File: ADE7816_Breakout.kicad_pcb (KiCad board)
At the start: 2 copper layers, 66 x 76.2 mm, 56 parts, among them J1 AudioJack3, J2 AudioJack3, J3 AudioJack3, J4 AudioJack3, J5 AudioJack3, J6 AudioJack3, J7 Barrel_Jack_Switch, J8 Conn_01x10, U1 ADE7816ACPZ, Y1 16.384MHz

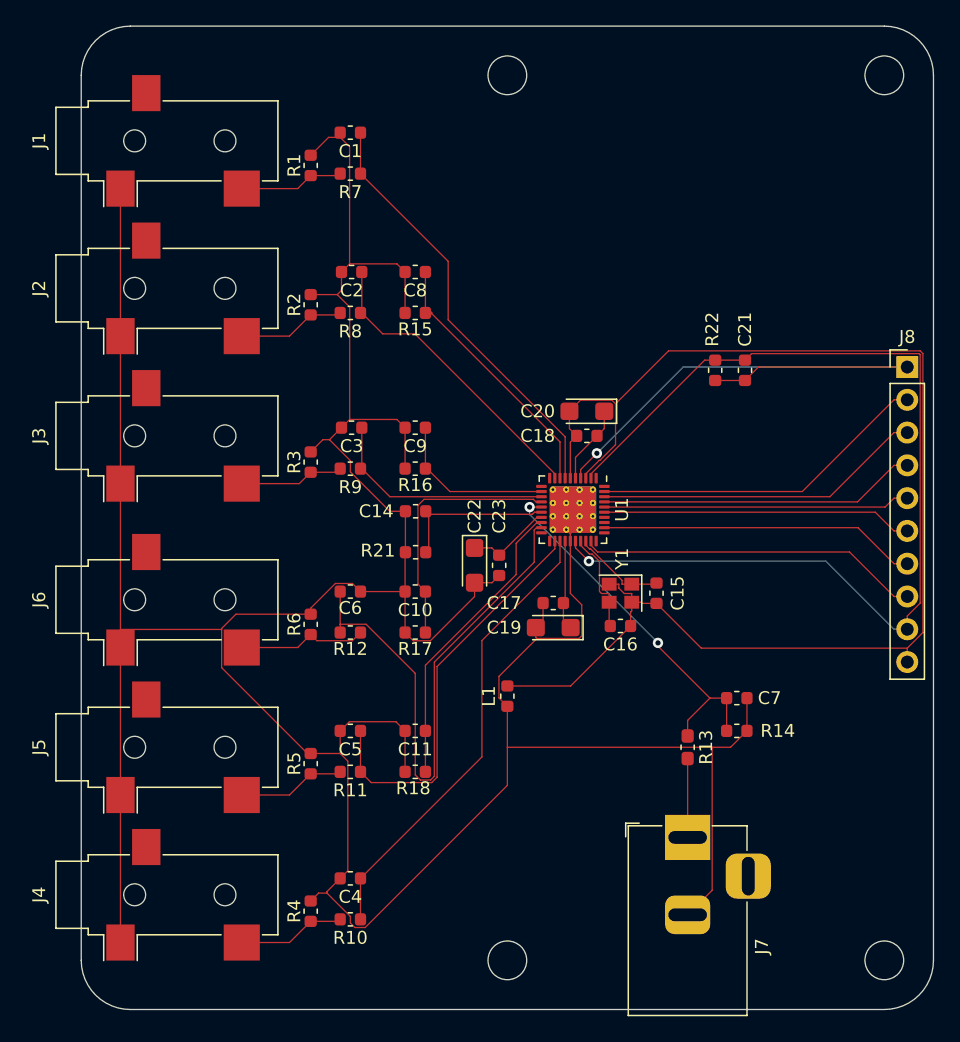
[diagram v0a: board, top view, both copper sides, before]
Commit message: Some routing
Signed-off-by: Tisham Dhar <whatnickd@gmail.com>
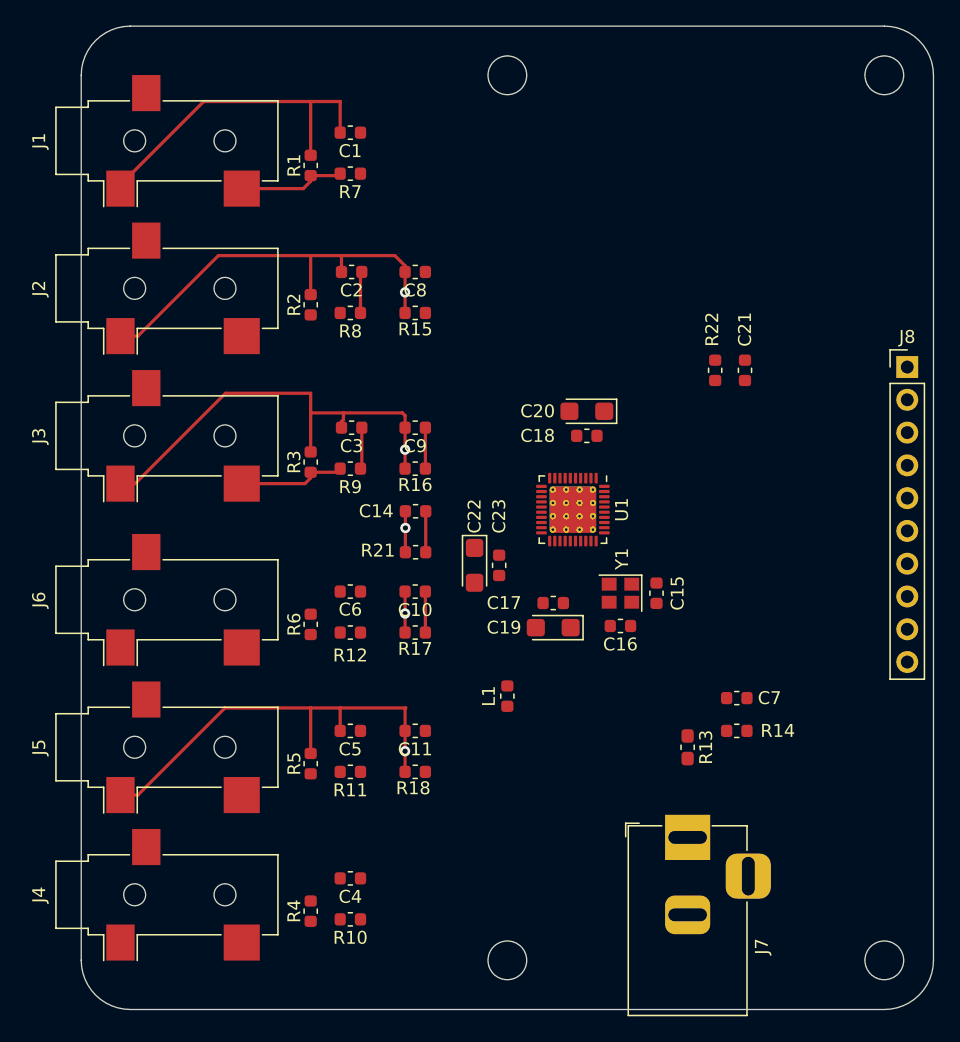
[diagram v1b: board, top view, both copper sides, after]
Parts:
- turned C6 to 180 degrees
- turned R12 to 180 degrees
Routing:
- net GNDA: track 296.7 -> 136.0 mm, vias 0 -> 5
- net GNDD: track 105.5 -> 0.00 mm
- net +3V3: track 80.3 -> 0.00 mm, vias 1 -> 0
- net /meter_module/~RESET: track 44.6 -> 0.00 mm, vias 1 -> 0
- net IFP: track 43.1 -> 0.00 mm
- net IDP: track 35.7 -> 0.00 mm
- net IAP: track 33.3 -> 0.00 mm
- net IEP: track 31.7 -> 0.00 mm
- net VP: track 29.0 -> 0.00 mm, vias 2 -> 0
- net /meter_module/~IRQ0: track 26.5 -> 0.00 mm
- net /meter_module/~CS: track 26.4 -> 0.00 mm
- net /meter_module/MOSI: track 25.5 -> 0.00 mm
- net /meter_module/MISO: track 24.6 -> 0.00 mm
- net /meter_module/~IRQ1: track 24.6 -> 0.00 mm
- net /meter_module/HSCLK: track 24.1 -> 0.00 mm
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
